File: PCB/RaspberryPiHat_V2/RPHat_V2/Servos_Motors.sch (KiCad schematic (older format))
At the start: 10 parts

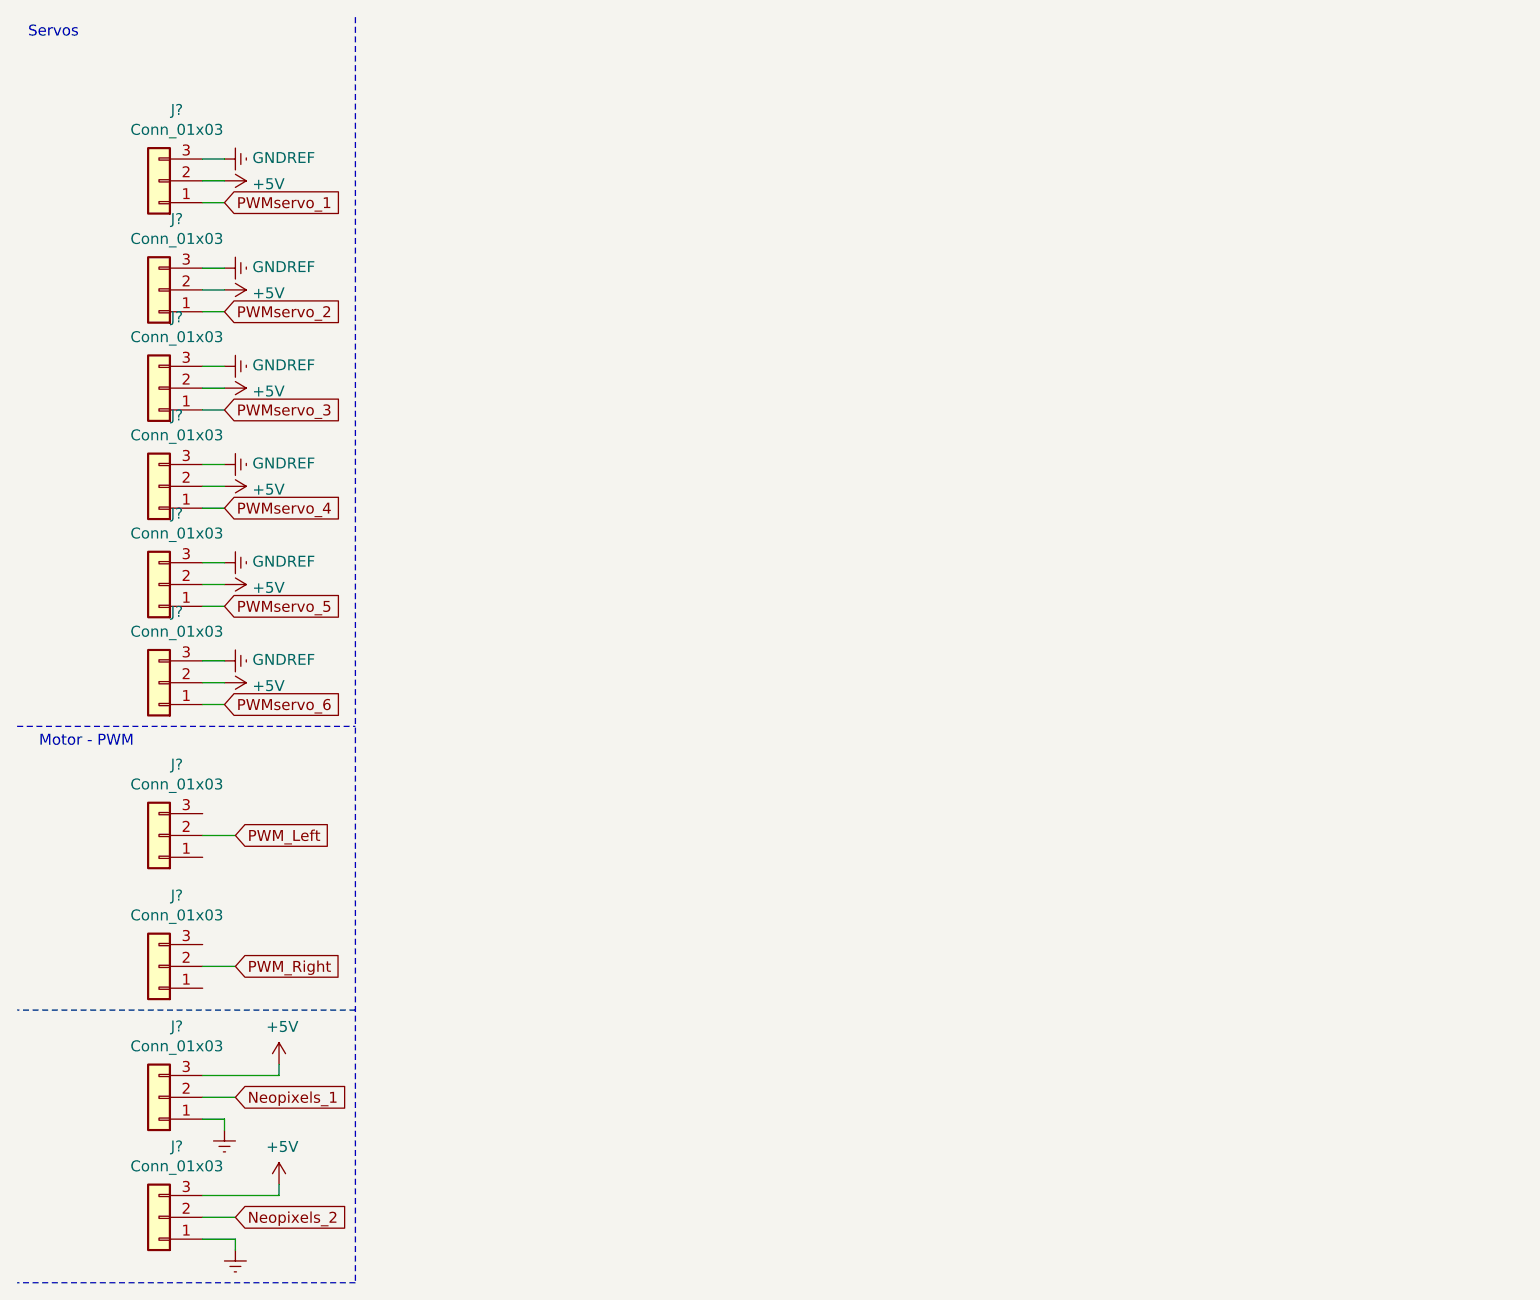
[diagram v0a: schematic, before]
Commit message: Schematic clean-up
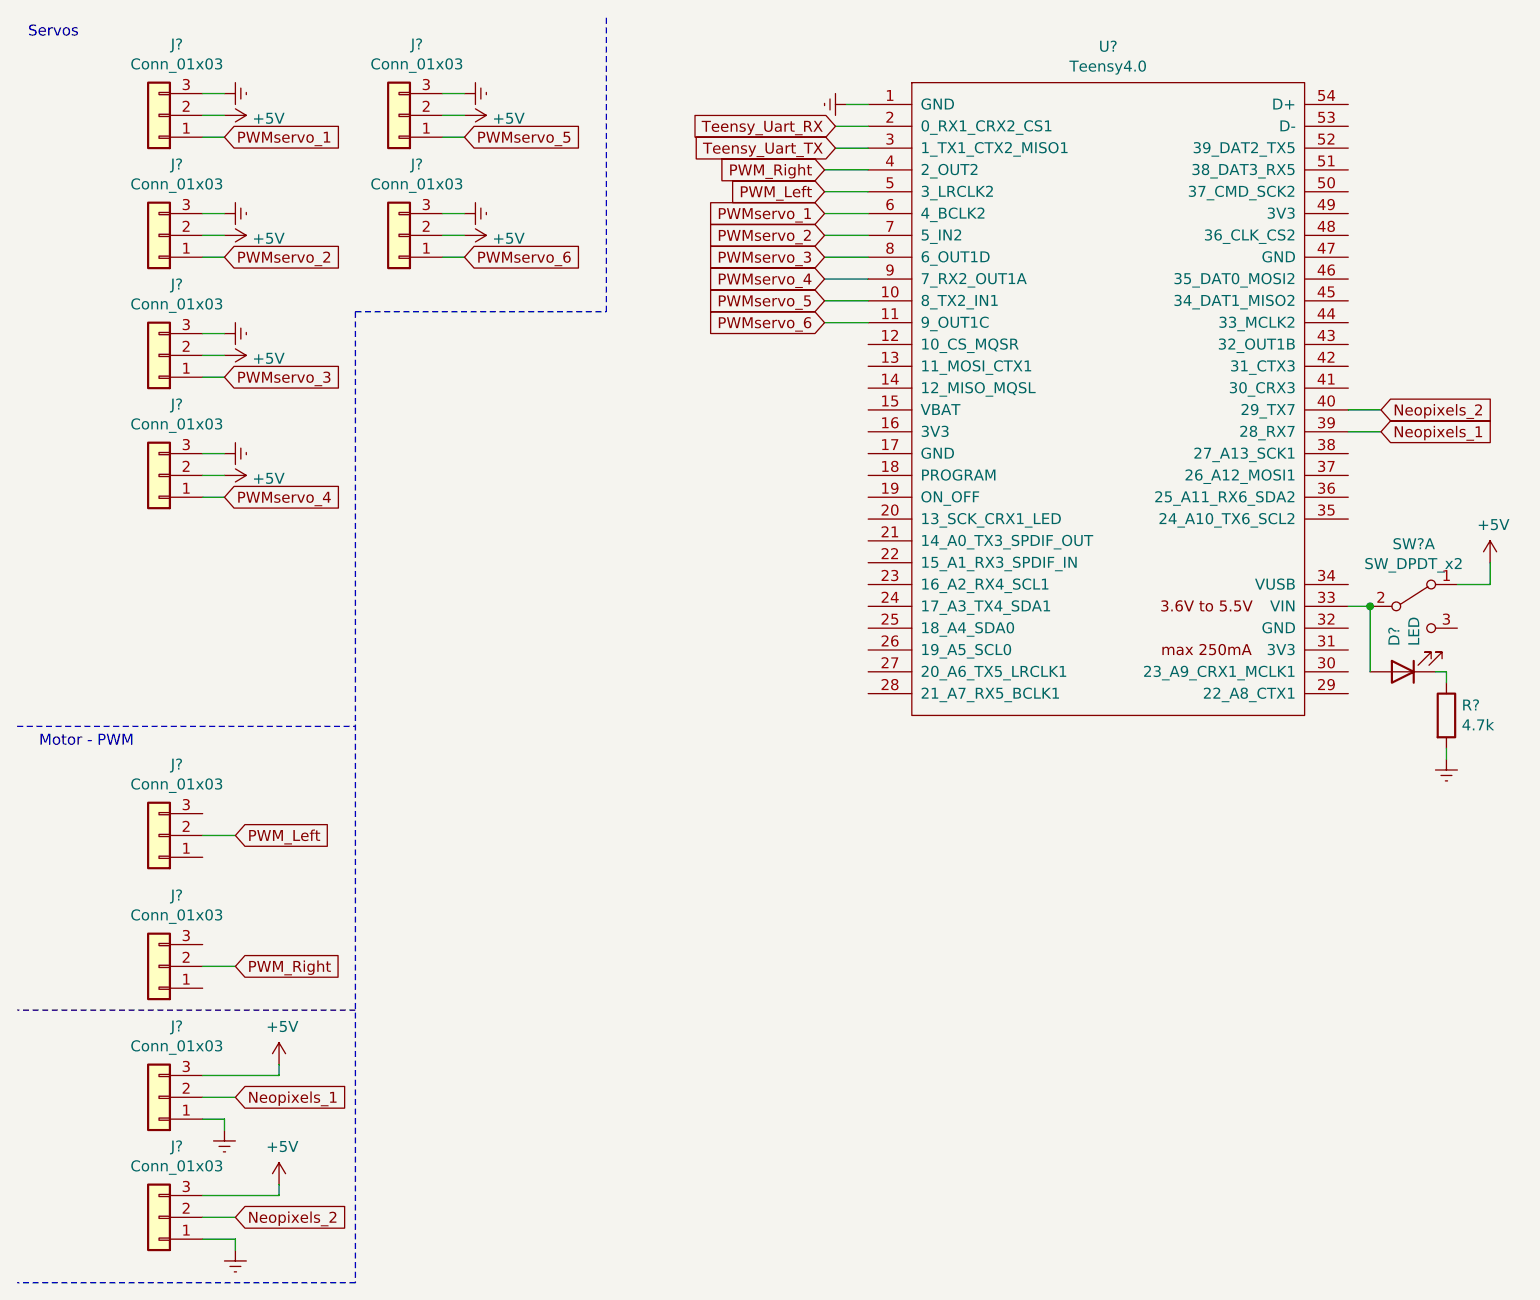
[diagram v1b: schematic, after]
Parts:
- added D?: LED, symbol Device:LED
- added R?: 4.7k, symbol Device:R
- added SW?: SW_DPDT_x2, symbol Switch:SW_DPDT_x2
- added U?: Teensy4.0, symbol RPHat_V2-rescue:Teensy4.0-teensy
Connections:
- net +5V: now also SW?.1 (A)
- net GNDREF: now also R?.2, U?.1 (GND)
- net Neopixels_1: now also U?.39 (28_RX7)
- net Neopixels_2: now also U?.40 (29_TX7)
- net PWM_Left: now also U?.5 (3_LRCLK2)
- net PWM_Right: now also U?.4 (2_OUT2)
- net PWMservo_1: now also U?.6 (4_BCLK2)
- net PWMservo_2: now also U?.7 (5_IN2)
- net PWMservo_3: now also U?.8 (6_OUT1D)
- net PWMservo_4: now also U?.9 (7_RX2_OUT1A)
- net PWMservo_5: now also U?.10 (8_TX2_IN1)
- net PWMservo_6: now also U?.11 (9_OUT1C)
- new net: D?.2 (A), SW?.2 (B), U?.33 (VIN)
- new net: D?.1 (K), R?.1
- new net Teensy_Uart_RX: U?.2 (0_RX1_CRX2_CS1)
- new net Teensy_Uart_TX: U?.3 (1_TX1_CTX2_MISO1)
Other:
- moved on the sheet: J?
